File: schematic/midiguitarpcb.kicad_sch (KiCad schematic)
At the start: 49 parts, among them CN1 NMJ6HCD2, J1 Conn_ARM_SWD_TagConnect_TC2030, J2 USB_C_Receptacle_USB2.0_16P, SW1 SW_Omron_B3FS, U1 DIN-504D-M5, U2 STM32H743VGTx, U3 AMS1117-3.3

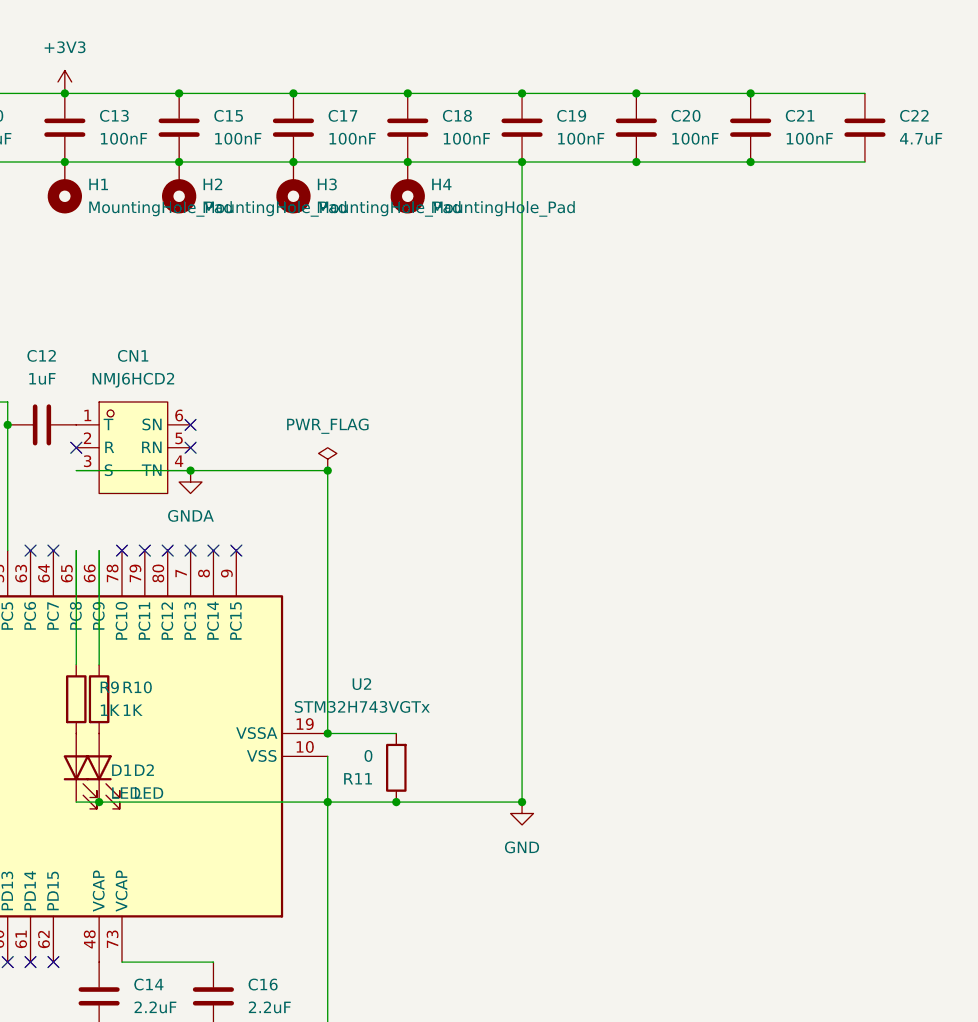
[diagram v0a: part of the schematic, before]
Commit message: skinny pcb
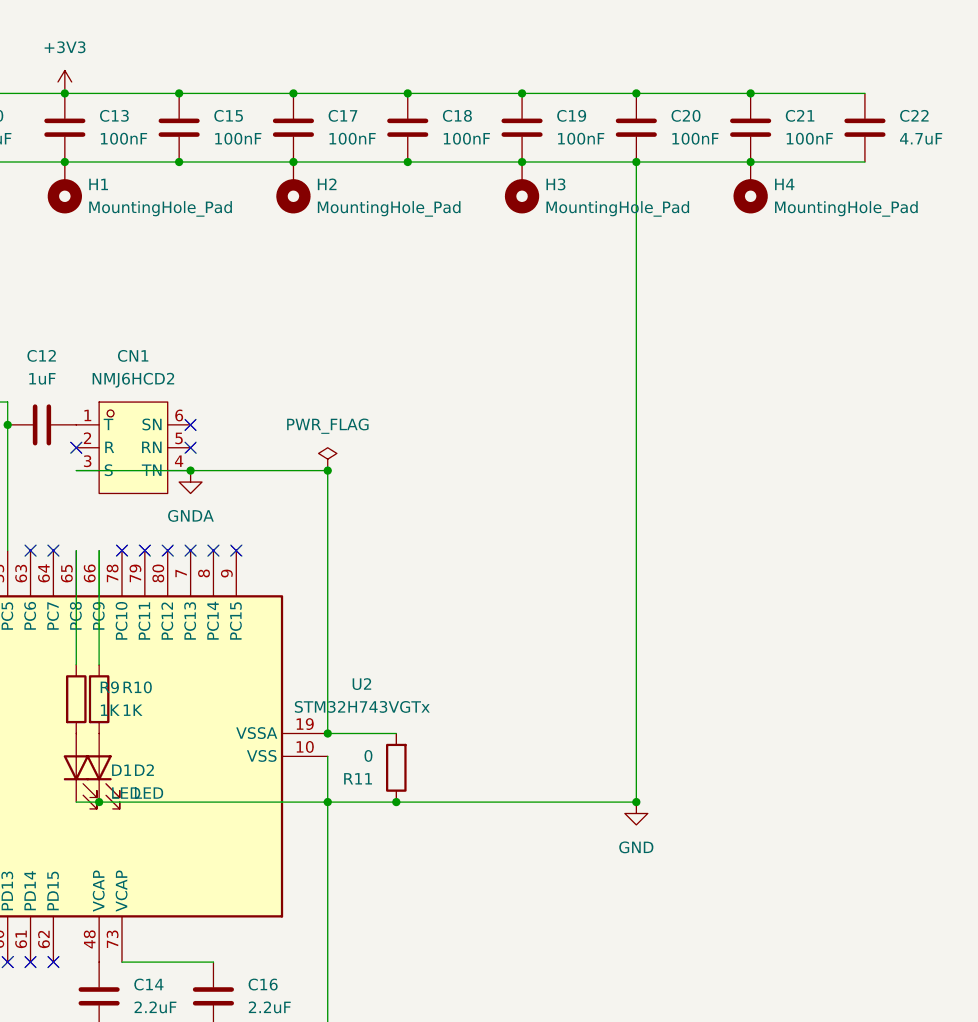
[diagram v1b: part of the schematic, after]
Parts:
- C1, C10, C11, C12, C13, C14, C15, C16, C17, C18, C19, C2, C20, C21, C22, C3, C4, C5, C6, C7, C8, C9: footprint Capacitor_SMD:C_0805_2012Metric -> Capacitor_SMD:C_0603_1608Metric
- D1, D2: footprint LED_SMD:LED_0805_2012Metric -> LED_SMD:LED_0603_1608Metric
- FB1, FB2, FB3: footprint Inductor_SMD:L_0805_2012Metric -> Inductor_SMD:L_0603_1608Metric
- R1, R10, R11, R2, R3, R4, R5, R6, R7, R8, R9: footprint Resistor_SMD:R_0805_2012Metric -> Resistor_SMD:R_0603_1608Metric
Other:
- moved on the sheet: H2, H3, H4
